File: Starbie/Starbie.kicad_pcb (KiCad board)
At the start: 2 copper layers, 140.6 x 97.3 mm, 18 parts, among them J1 Conn_01x04_Pin, J2 Conn_01x08_Pin, J3 Conn_01x02_Socket, SW1 SW_Push, SW2 SW_Push, SW3 SW_SPDT, U1 XIAO-ESP32-C3-SMD, U2 DHT11

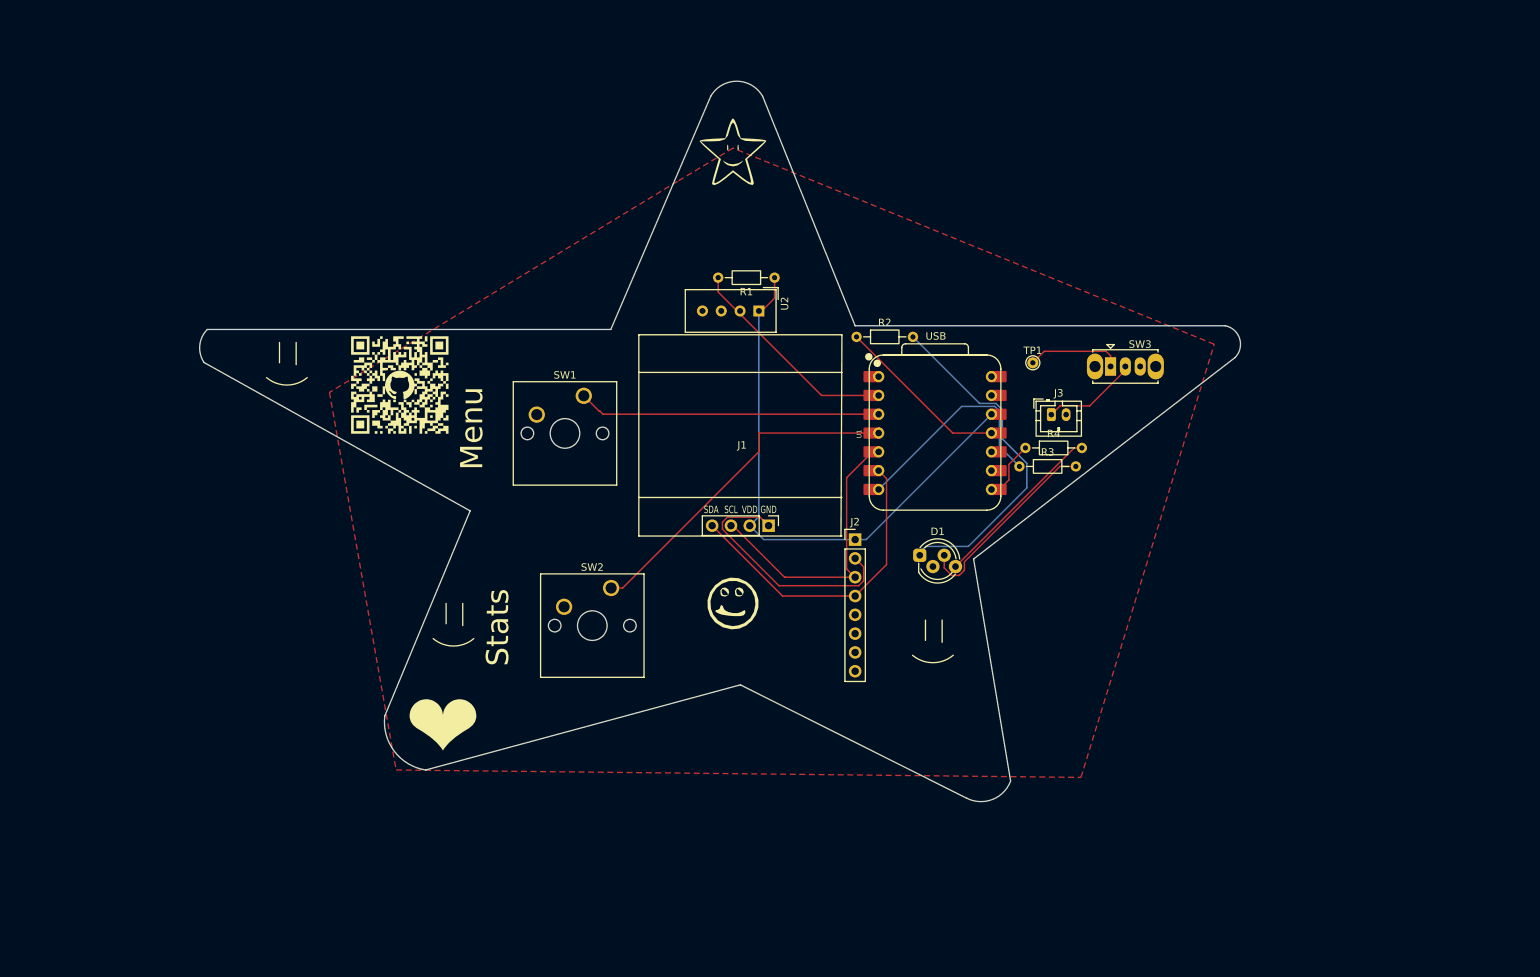
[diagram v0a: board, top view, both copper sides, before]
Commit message: bom. (WHY DID THIS TAKE SOOOO LONG)
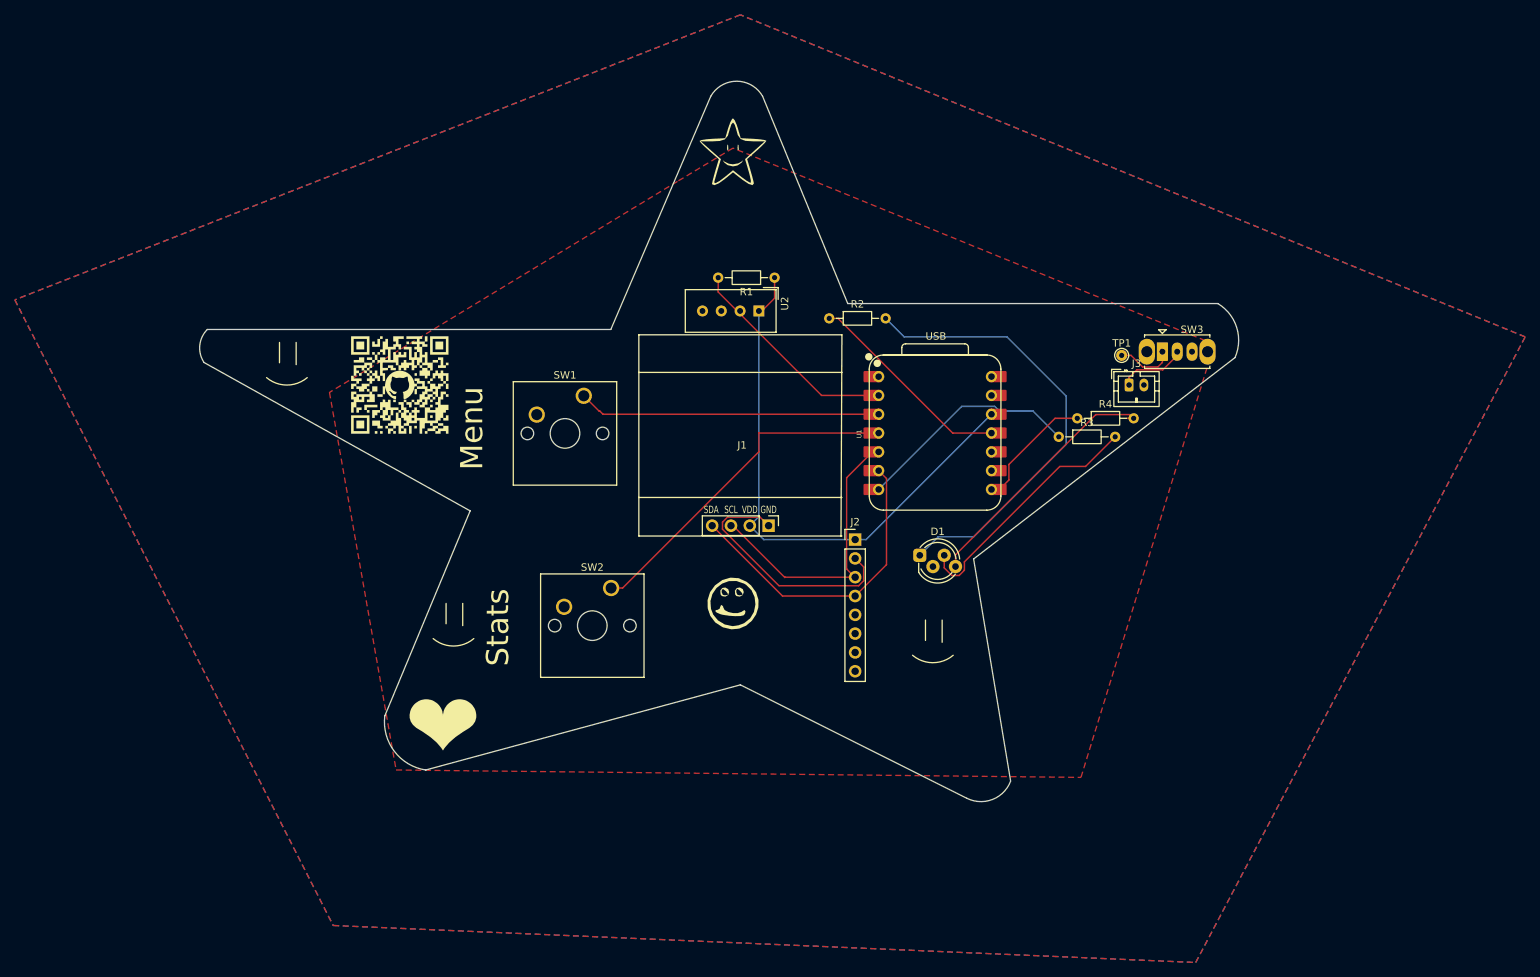
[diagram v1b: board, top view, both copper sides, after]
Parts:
- moved TP1 12.0 mm to (183.5, 77.0)
- moved J3 11.2 mm to (184.5, 81.0)
- moved R4 8.06 mm to (177.5, 85.5)
- moved SW3 7.28 mm to (189.0, 76.5)
- moved R3 6.65 mm to (175.0, 88.0)
- moved R2 4.46 mm to (144.0, 72.0)
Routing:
- net Net-(D1-RA): track 46.5 -> 61.2 mm
- net Net-(D1-BA): track 23.7 -> 34.7 mm
- net /LED_B: track 8.14 -> 16.8 mm
- net Net-(D1-GA): track 26.9 -> 33.9 mm
- net /VBAT_SW: track 12.8 -> 7.84 mm
- net /LED_R: track 23.6 -> 28.3 mm
- net /BAT_RAW: track 13.0 -> 9.24 mm
- net /LED_G: track 29.8 -> 30.7 mm
- added copper zone on B.Cu, net GND
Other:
- board size 140.6 x 97.3 mm -> 140.3 x 97.3 mm
